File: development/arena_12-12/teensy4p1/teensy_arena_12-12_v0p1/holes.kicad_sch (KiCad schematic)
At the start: 4 parts

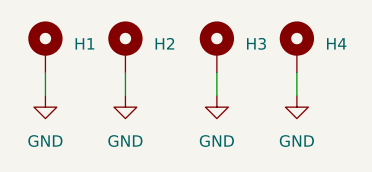
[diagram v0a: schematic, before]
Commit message: bump buffer version to 0.2
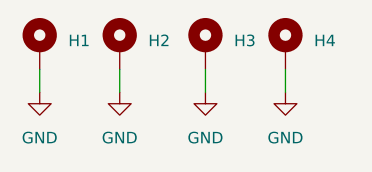
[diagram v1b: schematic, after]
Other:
- moved on the sheet: H1, H2, H3, H4
